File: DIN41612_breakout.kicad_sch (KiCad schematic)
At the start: 4 parts, among them J1 09031967921

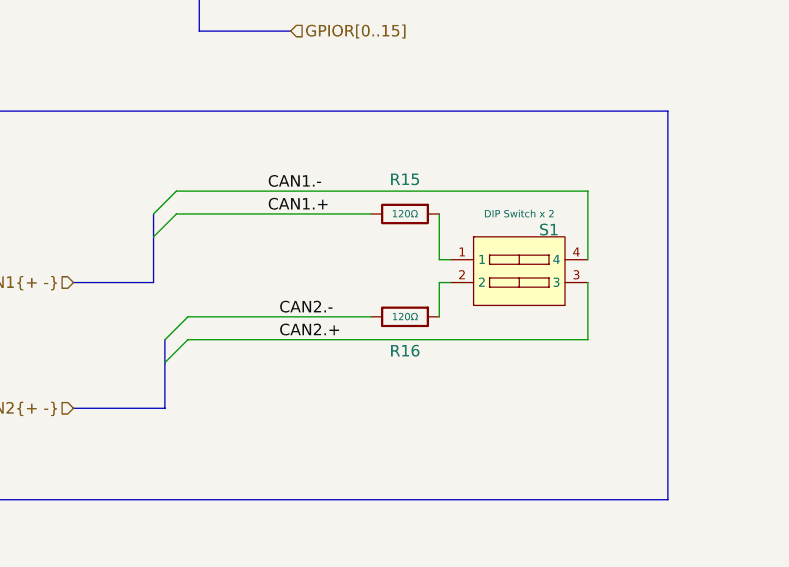
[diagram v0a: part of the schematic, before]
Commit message: Change schematic
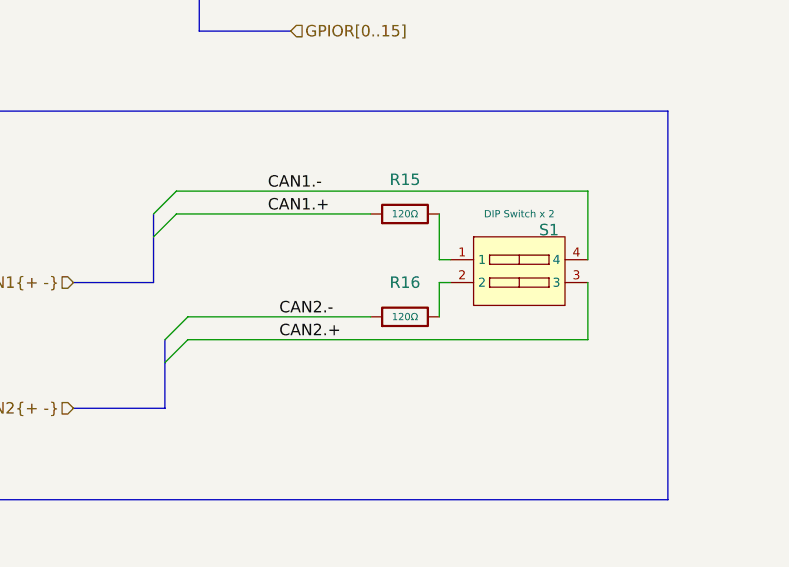
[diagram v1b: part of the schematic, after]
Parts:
- removed R15, R16: 120Ω, PCM_JLCPCB:R_1206, symbol PCM_JLCPCB-Resistors:1206,120Ω
- added R15, R16: 120Ω, PCM_JLCPCB:R_0603, symbol PCM_JLCPCB-Resistors:0603,120Ω
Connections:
- net CAN1.+: now also R15.1
- net CAN2.-: now also R16.1
- net at S1.2: now also R16.2
- net at S1.1: now also R15.2
